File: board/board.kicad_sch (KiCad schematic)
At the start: 1 part

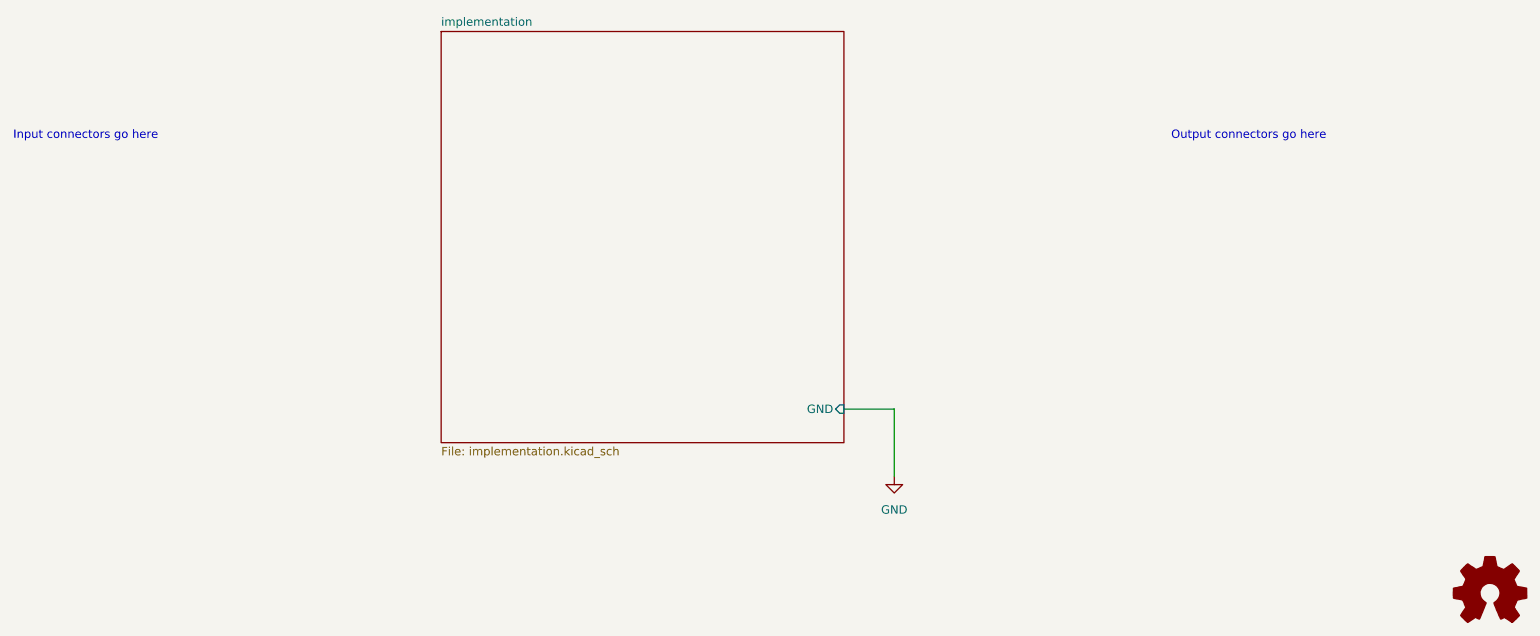
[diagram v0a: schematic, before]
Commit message: initial
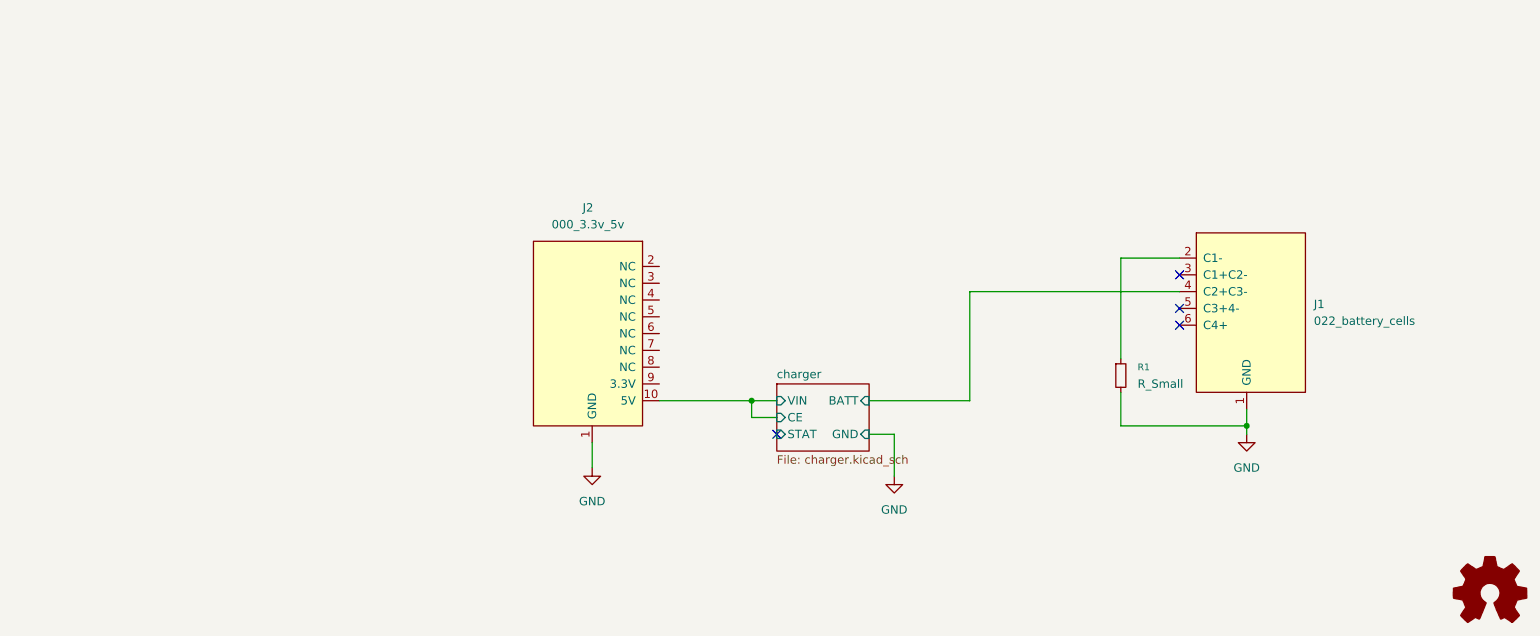
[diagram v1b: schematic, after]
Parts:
- added J1: 022_battery_cells, on_edge:on_edge_2x05_host, symbol put_on_edge:022_battery_cells
- added J2: 000_3.3v_5v, on_edge:on_edge_2x05_device, symbol put_on_edge:000_3.3v_5v
- added R1: R_Small, symbol Device:R_Small
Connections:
- net GND: now also J1.1 (GND), J2.1 (GND), R1.2
- new net: J1.2 (C1-), R1.1
- new net charger/BATT: J1.4 (C2+C3-)
- new net charger/CE: J2.10 (5V)
- no-connect marks 0 -> 4
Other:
- sheet implementation renamed charger
- sheet charger: file implementation.kicad_sch -> charger.kicad_sch
- sheet charger ports: added BATT, CE, STAT, VIN; removed none
- note removed: "Input connectors go here"
- note removed: "Output connectors go here"
